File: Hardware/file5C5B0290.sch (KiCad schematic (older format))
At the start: 44 parts, among them J15 Conn_02x05_Odd_Even, U10 TPS82140, U11 TPS82140, U12 TPSM84209RKHT, U9 TPS82140

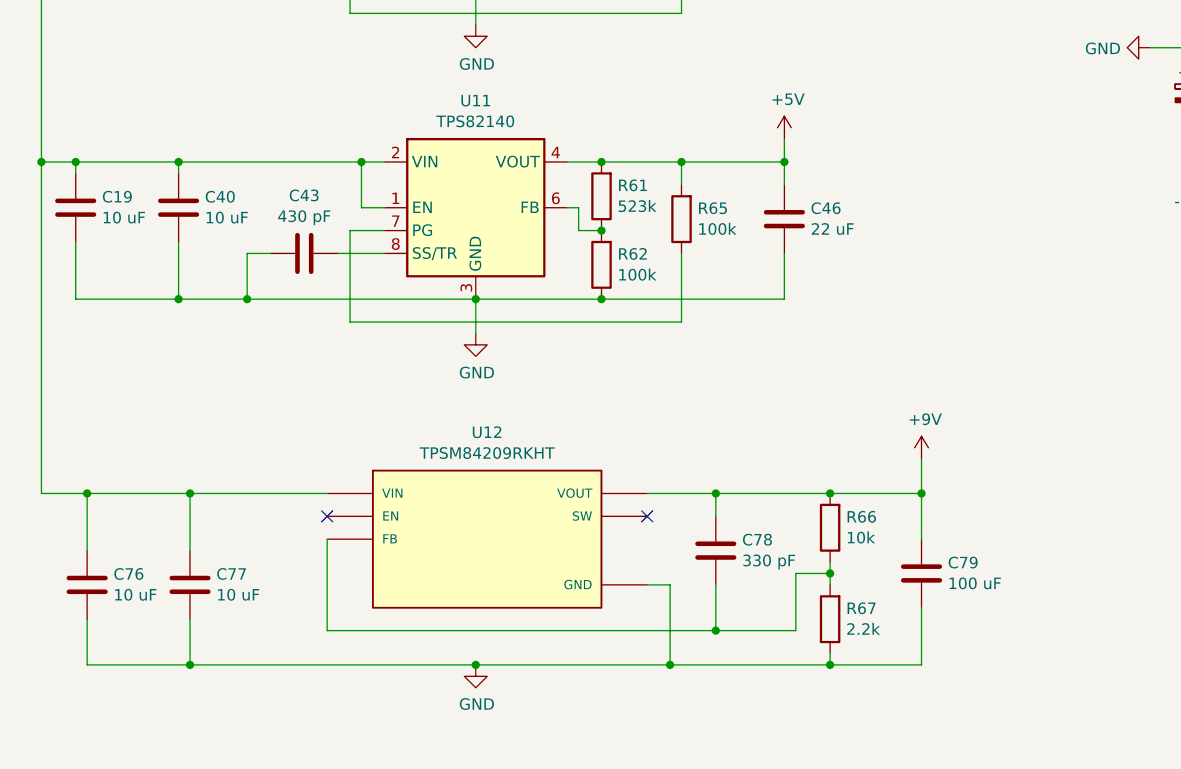
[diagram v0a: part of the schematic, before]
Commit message: Started state machine
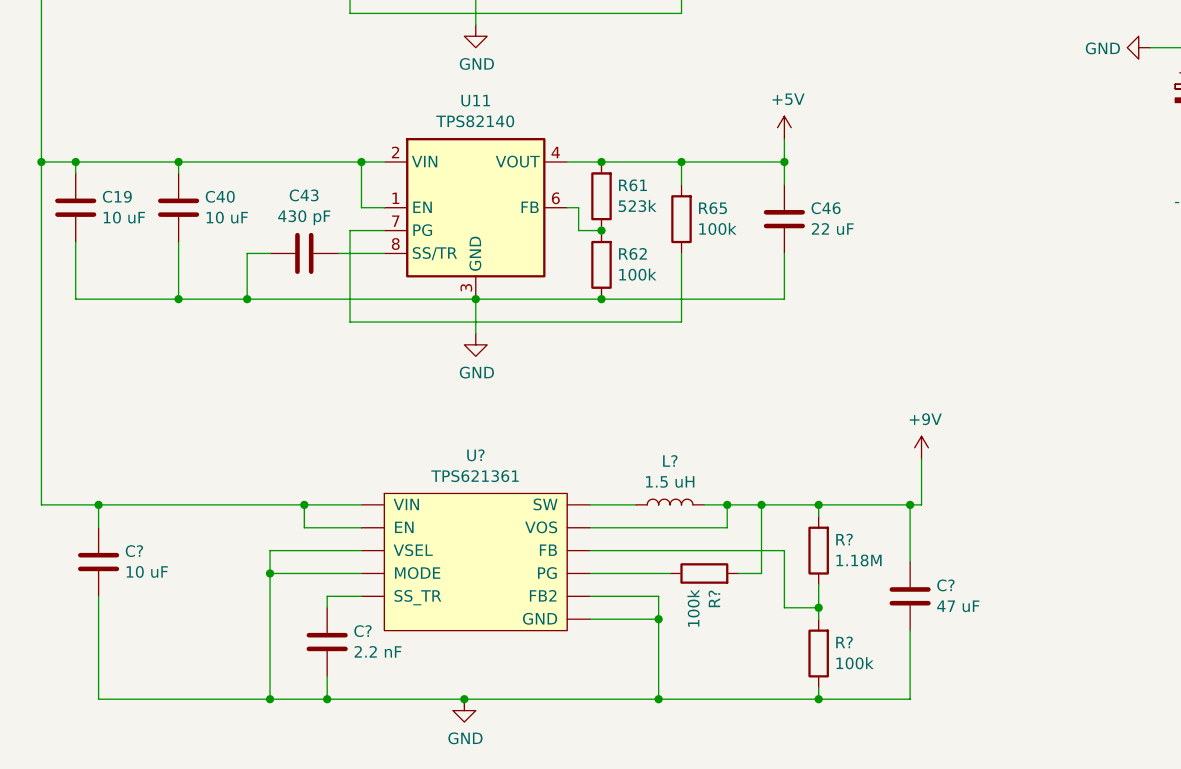
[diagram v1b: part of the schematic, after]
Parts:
- removed C76, C77: 10 uF, Capacitor_SMD:C_0603_1608Metric, symbol Device:C
- removed C78: 330 pF, Capacitor_SMD:C_0603_1608Metric, symbol Device:C
- removed C79: 100 uF, Capacitor_SMD:C_0603_1608Metric, symbol Device:C
- removed R66: 10k, Resistor_SMD:R_0603_1608Metric, symbol Device:R
- removed R67: 2.2k, Resistor_SMD:R_0603_1608Metric, symbol Device:R
- removed U12: TPSM84209RKHT, TPSM84209RKHT:VREG_TPSM84209RKHT, symbol TPSM84209RKHT:TPSM84209RKHT
- added C?: 10 uF, Capacitor_SMD:C_0603_1608Metric, symbol Device:C
- added C?: 2.2 nF, Capacitor_SMD:C_0603_1608Metric, symbol Device:C
- added C?: 47 uF, Capacitor_SMD:C_0603_1608Metric, symbol Device:C
- added L?: 1.5 uH, symbol Device:L
- added R? (x2): 100k, Resistor_SMD:R_0603_1608Metric, symbol Device:R
- added R?: 1.18M, Resistor_SMD:R_0603_1608Metric, symbol Device:R
- added U?: TPS621361, symbol Regulator_Switching:TPS621361
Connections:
- net +12V: now also C?.1, U?.1 (VIN), U?.8 (EN)
- net +9V: now also C?.1, L?.2, R?.2, R?.2, U?.6 (VOS)
- net GND: now also C?.2, C?.2, C?.2, R?.1, U?.10 (MODE), U?.11 (VSEL), U?.3 (GND), U?.4 (FB2)
- new net: L?.1, U?.2 (SW)
- new net: R?.1, R?.2, U?.5 (FB)
- new net: R?.1, U?.7 (PG)
- new net: C?.1, U?.9 (SS_TR)
- no-connect marks 2 -> 0
